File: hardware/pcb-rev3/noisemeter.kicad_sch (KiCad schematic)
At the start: 18 parts, among them J1 USB_B_Micro, SW1 SW_Push, U1 AP2112K-3.3, U2 ESP32-C3-MINI-1-N4

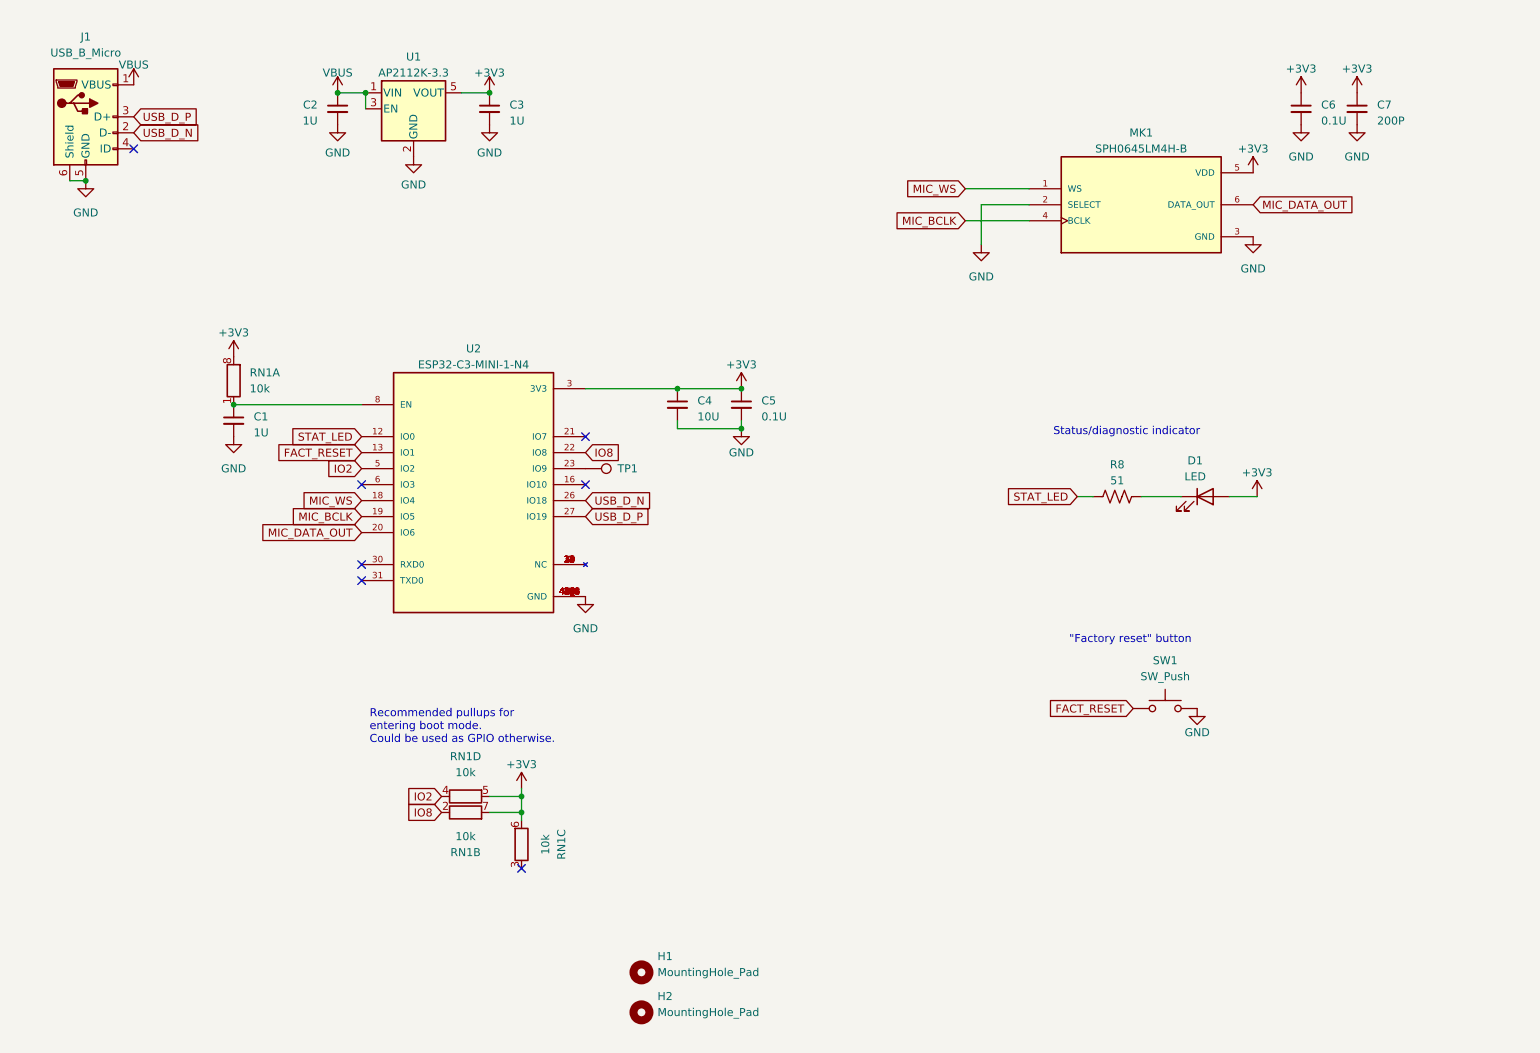
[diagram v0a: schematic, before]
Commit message: cleaning up layout
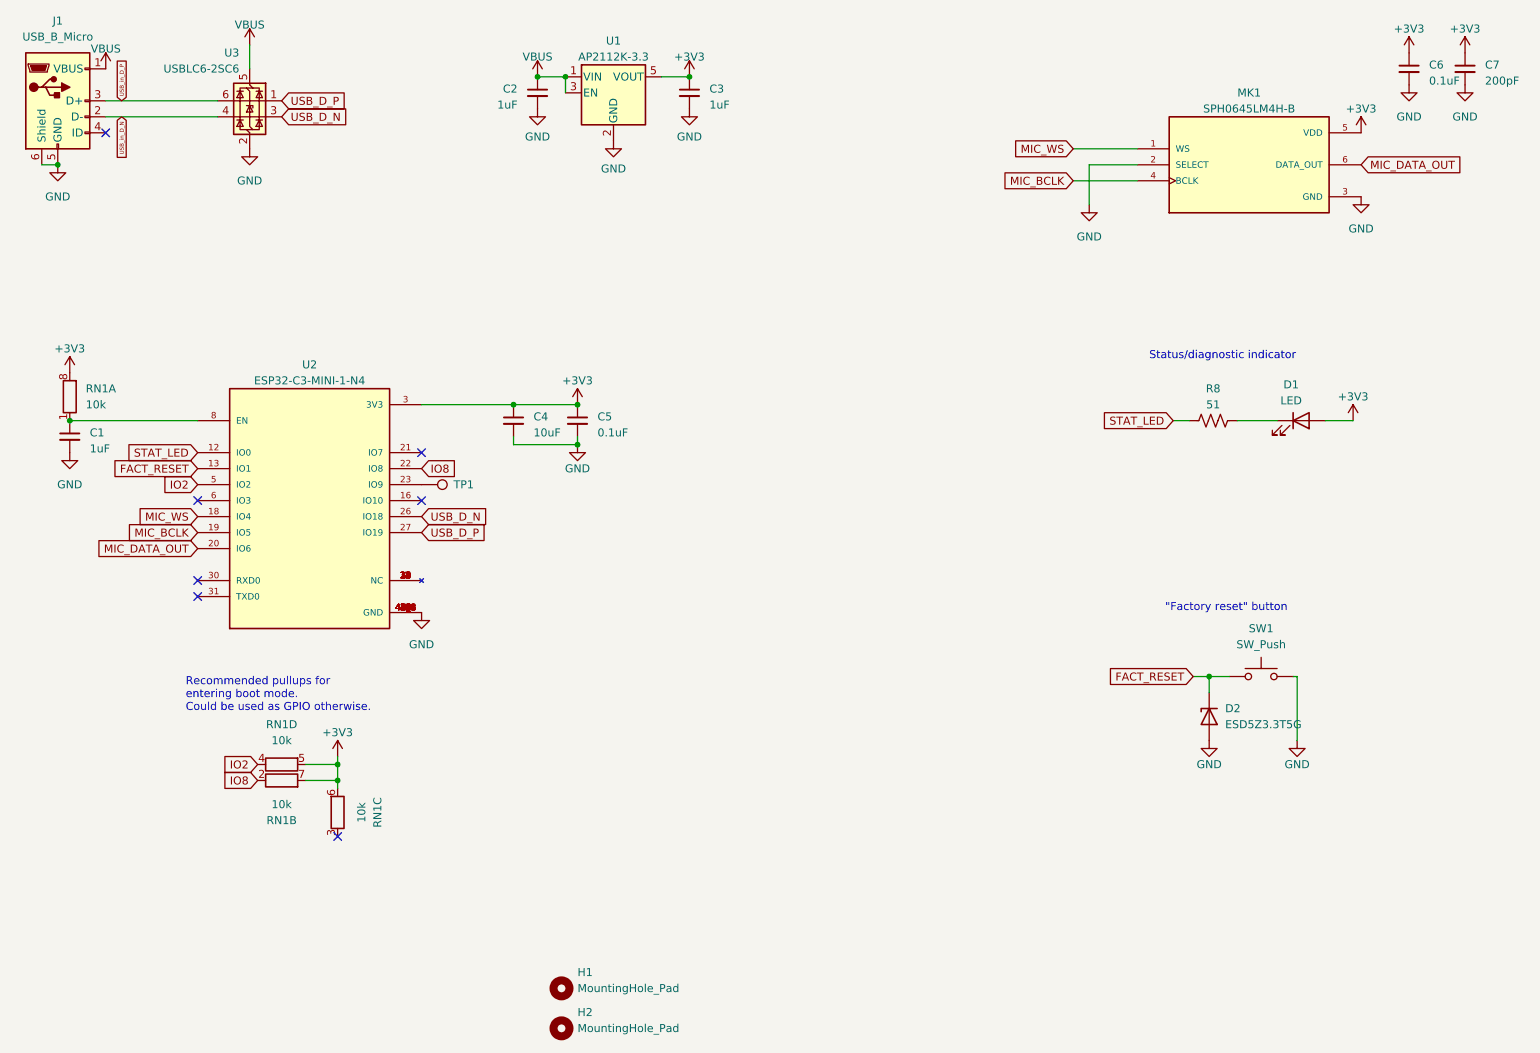
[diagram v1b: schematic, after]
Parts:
- added D2: ESD5Z3.3T5G, Diode_SMD:D_0603_1608Metric, symbol Diode:ESD5Zxx
- added U3: USBLC6-2SC6, Package_TO_SOT_SMD:SOT-23-6, symbol Power_Protection:USBLC6-2SC6
- C1, C2, C3: value 1U -> 1uF; Part Number CC0603KRX5R6BB105 -> CC0603KRX7R7BB105
- C4: value 10U -> 10uF; Part Number CL21A106KPFNNNG -> CL21A106KOQNNNE
- C5, C6: value 0.1U -> 0.1uF
- C7: value 200P -> 200pF; Part Number 06033A201FAT2A -> CL10B201KB8NNNC
- RN1: Part Number (none) -> CAY16-103J4LF
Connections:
- net FACT_RESET: now also D2.1 (K)
- net GND: now also D2.2 (A), U3.2 (GND)
- net USB_D_N: now also U3.3 (I/O2); no longer J1.2 (D-)
- net USB_D_P: now also U3.1 (I/O1); no longer J1.3 (D+)
- net VBUS: now also U3.5 (VBUS)
- new net USB_in_D_N: J1.2 (D-), U3.4 (I/O2)
- new net USB_in_D_P: J1.3 (D+), U3.6 (I/O1)
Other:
- moved on the sheet: C1, C2, C3, C4, C5, C6, C7, D1, H1, H2, J1, MK1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
